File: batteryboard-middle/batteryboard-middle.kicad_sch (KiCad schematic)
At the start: 7 parts, among them J1 Conn 02x10 1.27mm, J2 Conn_01x02, J3 Conn_01x02

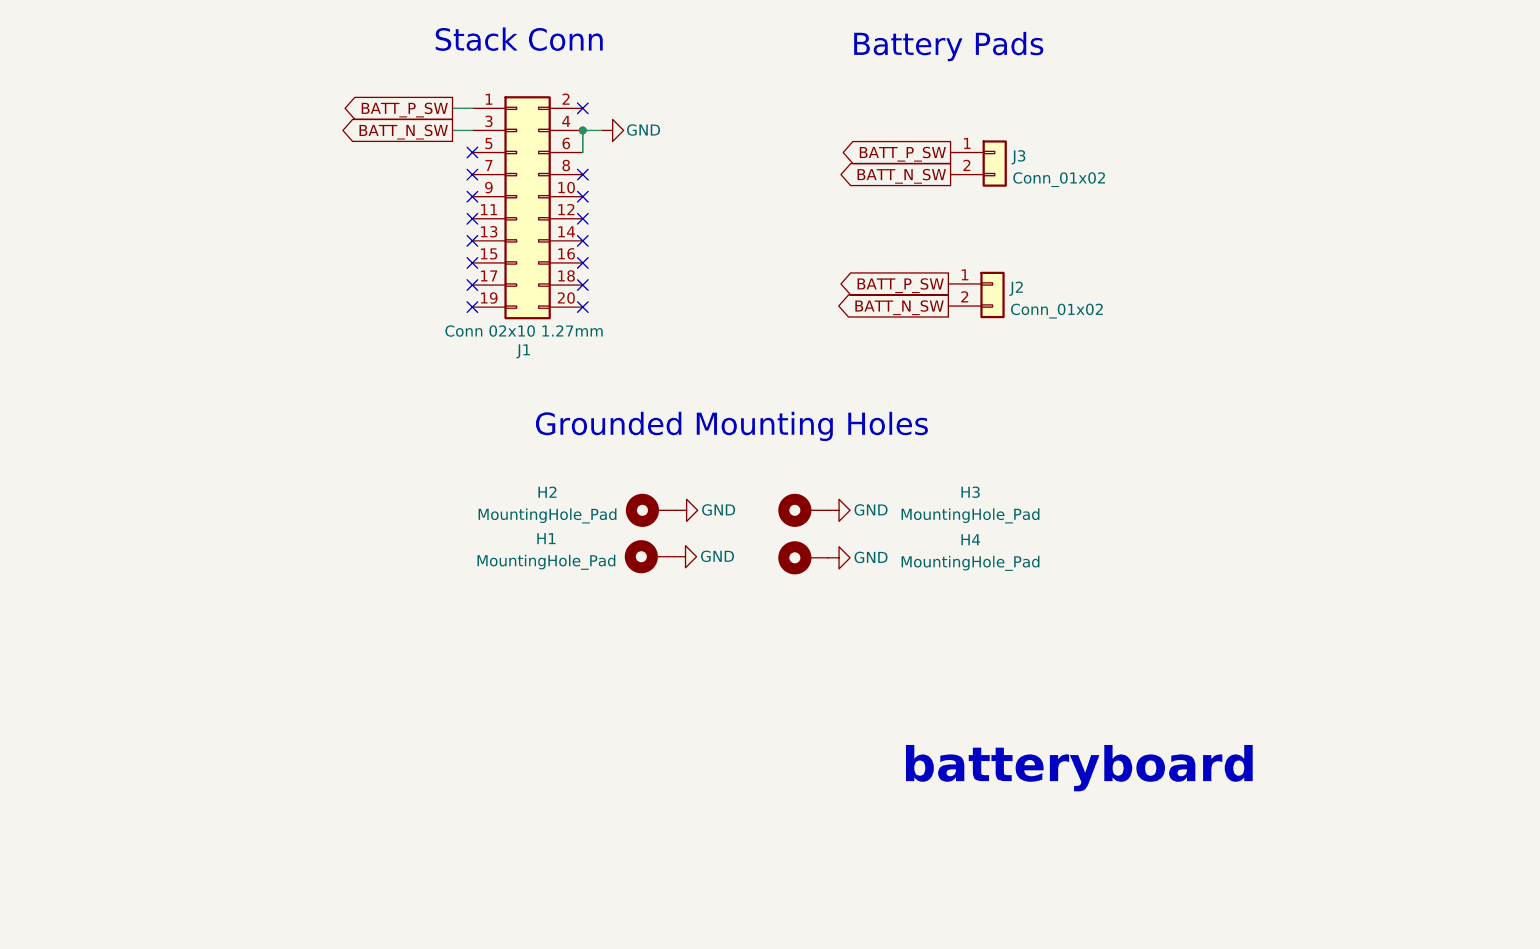
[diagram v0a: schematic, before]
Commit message: modified connector arrangement
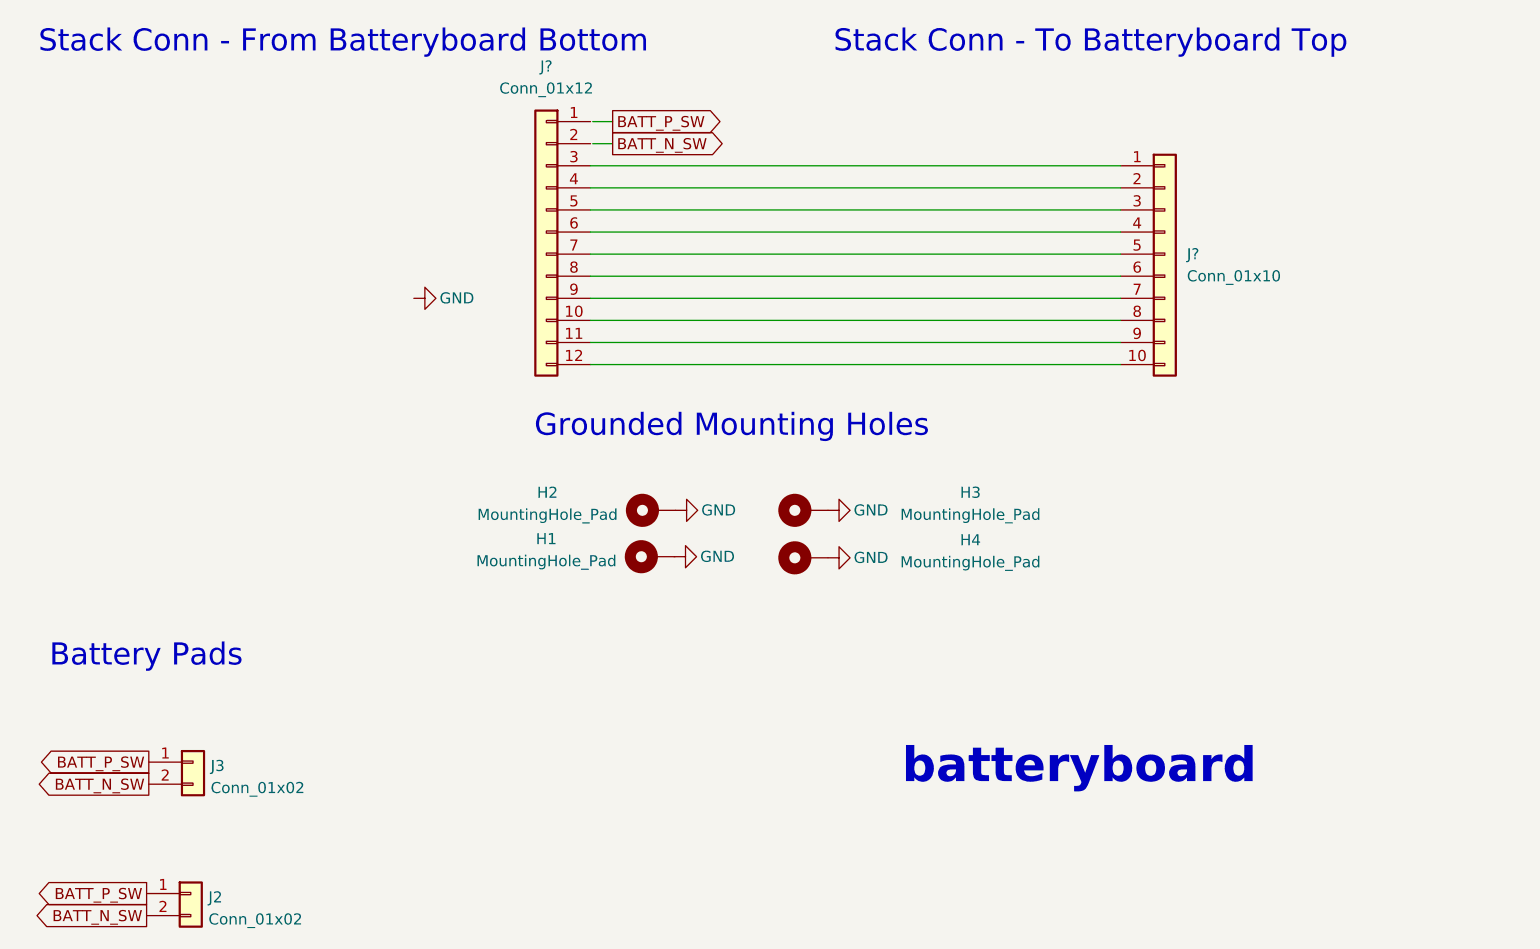
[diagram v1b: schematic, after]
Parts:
- removed J1: Conn 02x10 1.27mm, Connector_PinHeader_1.27mm:PinHeader_2x10_P1.27mm_Vertical, symbol Connector_Generic:Conn_02x10_Odd_Even
- added J?: Conn_01x12, symbol Connector_Generic:Conn_01x12
- added J?: Conn_01x10, symbol Connector_Generic:Conn_01x10
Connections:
- new net: J?.10 (Pin_10), J?.8 (Pin_8)
- new net: J?.11 (Pin_11), J?.9 (Pin_9)
- new net: J?.10 (Pin_10), J?.12 (Pin_12)
- new net: J?.1 (Pin_1), J?.3 (Pin_3)
- new net: J?.2 (Pin_2), J?.4 (Pin_4)
- new net: J?.3 (Pin_3), J?.5 (Pin_5)
- new net: J?.4 (Pin_4), J?.6 (Pin_6)
- new net: J?.5 (Pin_5), J?.7 (Pin_7)
- new net: J?.6 (Pin_6), J?.8 (Pin_8)
- new net: J?.7 (Pin_7), J?.9 (Pin_9)
- no-connect marks 16 -> 0
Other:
- note added: "Stack Conn - From Batteryboard Bottom"
- note added: "Stack Conn - To Batteryboard Top"
- note removed: "Stack Conn"
- moved on the sheet: J2, J3
